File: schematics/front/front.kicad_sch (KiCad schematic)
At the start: 36 parts, among them J1 USB_B_Micro, J2 MOTOR, J3 Conn_01x08_Pin, J6 Conn_02x04_Odd_Even, SW1 RESET, SW2 BOOT, SW3 MODE, U1 LD1117AG-33-AA3-A-R, U2 ESP32-S2-MINI-2-N4, U3 DRV8836

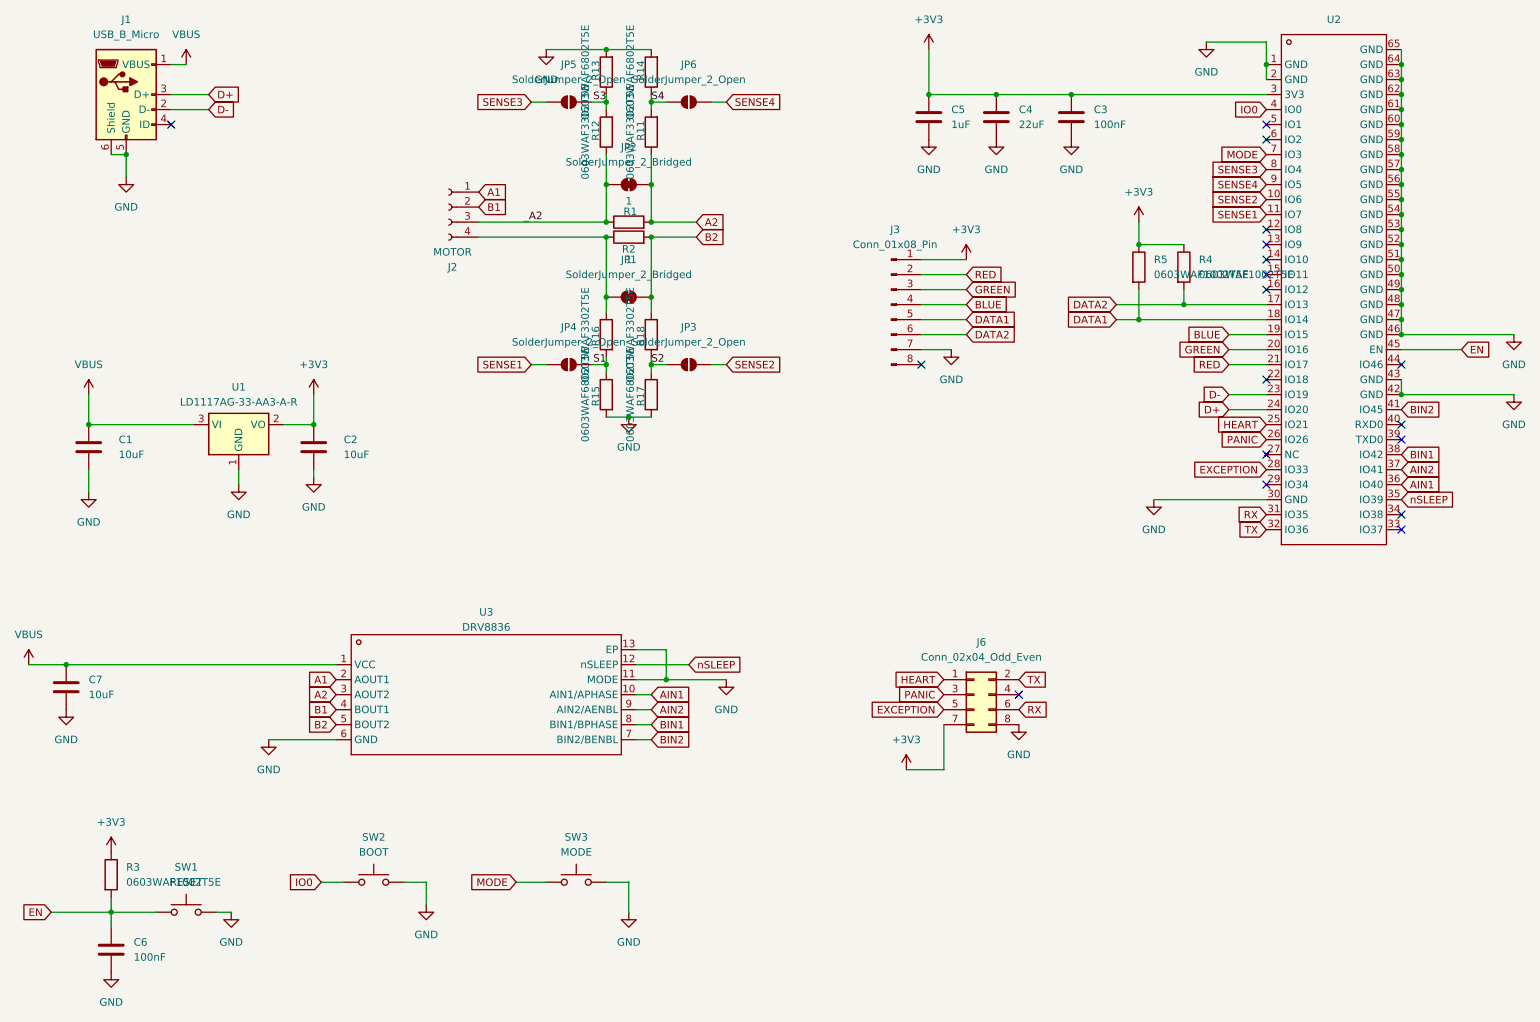
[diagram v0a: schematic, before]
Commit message: Signed-off-by: Ray33ee <30669752+ray33ee@users.noreply.github.com>
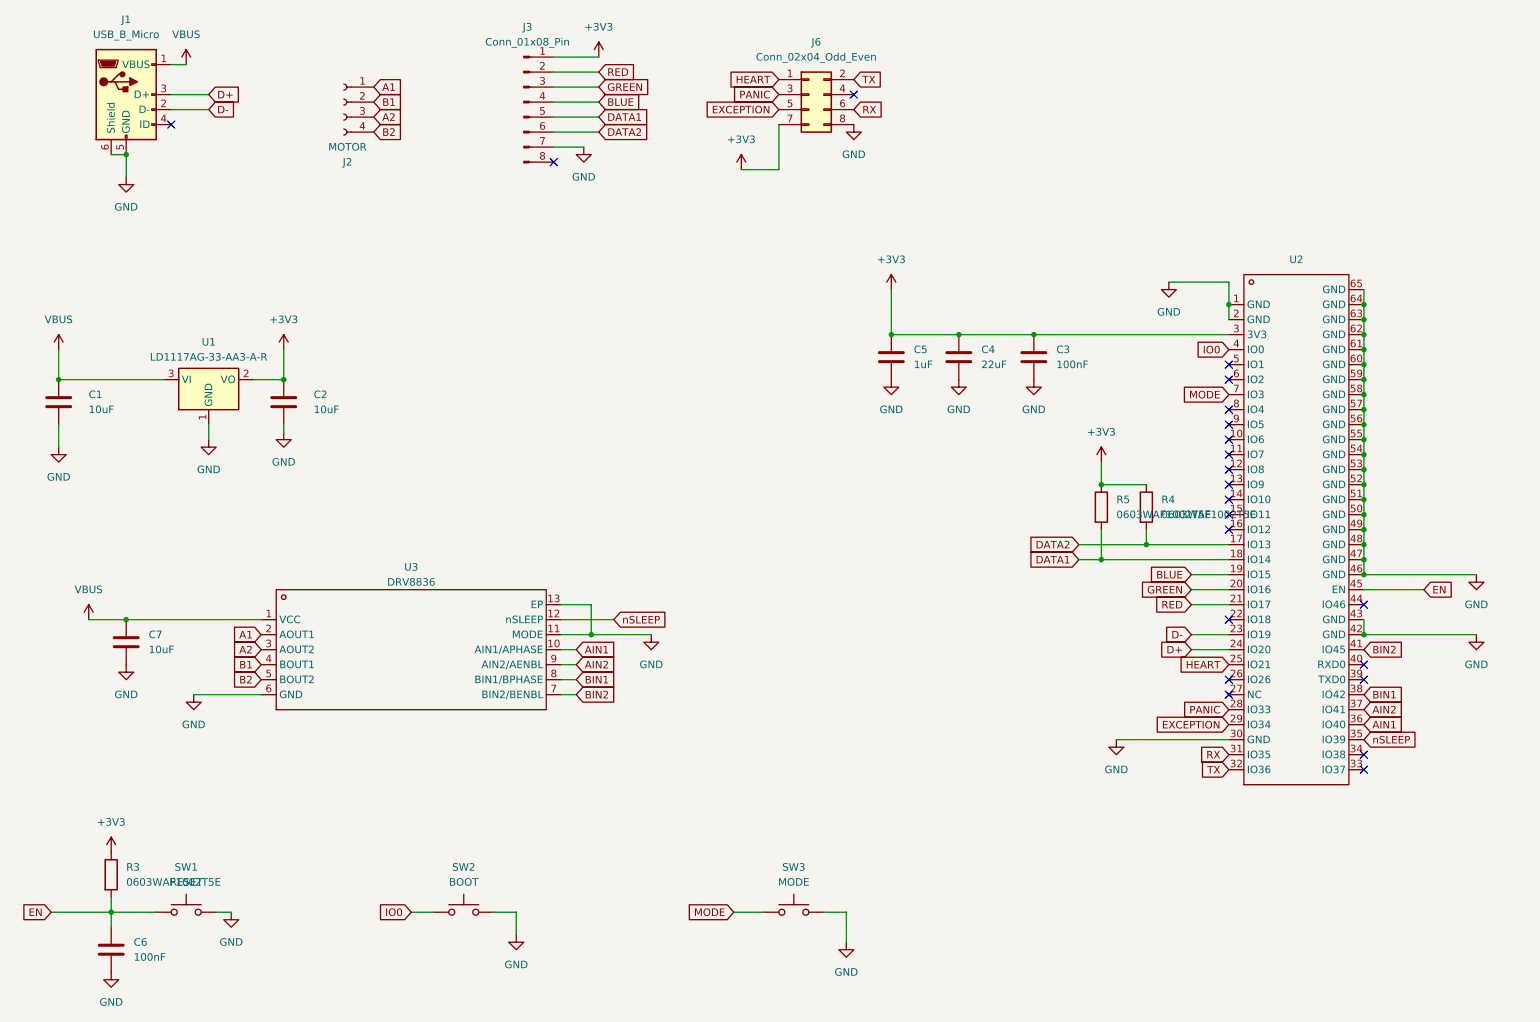
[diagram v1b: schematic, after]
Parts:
- removed JP1, JP2: SolderJumper_2_Bridged, Jumper:SolderJumper-2_P1.3mm_Bridged_RoundedPad1.0x1.5mm, symbol Jumper:SolderJumper_2_Bridged
- removed JP3, JP4, JP5, JP6: SolderJumper_2_Open, Jumper:SolderJumper-2_P1.3mm_Open_RoundedPad1.0x1.5mm, symbol Jumper:SolderJumper_2_Open
- removed R1, R2: 1, Resistor_SMD:R_1206_3216Metric_Pad1.30x1.75mm_HandSolder, symbol Device:R
- removed R11, R12, R16, R18: 0603WAF3302T5E, Resistor_SMD:R_0603_1608Metric, symbol Device:R
- removed R13, R14, R15, R17: 0603WAF6802T5E, Resistor_SMD:R_0603_1608Metric, symbol Device:R
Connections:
- net _A2 is gone; now on net A2: J2.3 (Pin_3)
- net B2: now also J2.4 (Pin_4)
- net EXCEPTION: now also U2.29 (IO34); no longer U2.28 (IO33)
- net PANIC: now also U2.28 (IO33); no longer U2.26 (IO26)
- net SENSE1: no longer names the net of U2.11 (IO7)
- net SENSE2: no longer names the net of U2.10 (IO6)
- net SENSE3: no longer names the net of U2.8 (IO4)
- net SENSE4: no longer names the net of U2.9 (IO5)
- no-connect marks 18 -> 22
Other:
- moved on the sheet: C1, C2, C3, C4, C5, C7, J2, J3, J6, R4, R5, SW2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
